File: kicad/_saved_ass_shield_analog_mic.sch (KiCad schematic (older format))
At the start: 151 parts, among them J1 6-40V, J2 DEBUG, J3 5V, J4 UART2, J5 U.FL, J6 i2s, J7 SP, J8 U.FL, M1 CR1220SMD, Q1 BC817, U1 OPiZero, U2 DS3231M, U3 24LC256, U4 nRF24L01P, U5 PCF8574, U6 CC2530F, X1 USB_F1, X2 USB_F1, Y1 9,84375 MHz, Y2 13,5600 MHz, Y3 4,8970 MHz, Y4 6,7458 MHz, Y5 32 MHz, Y6 16 MHz, Y7 32 MHz

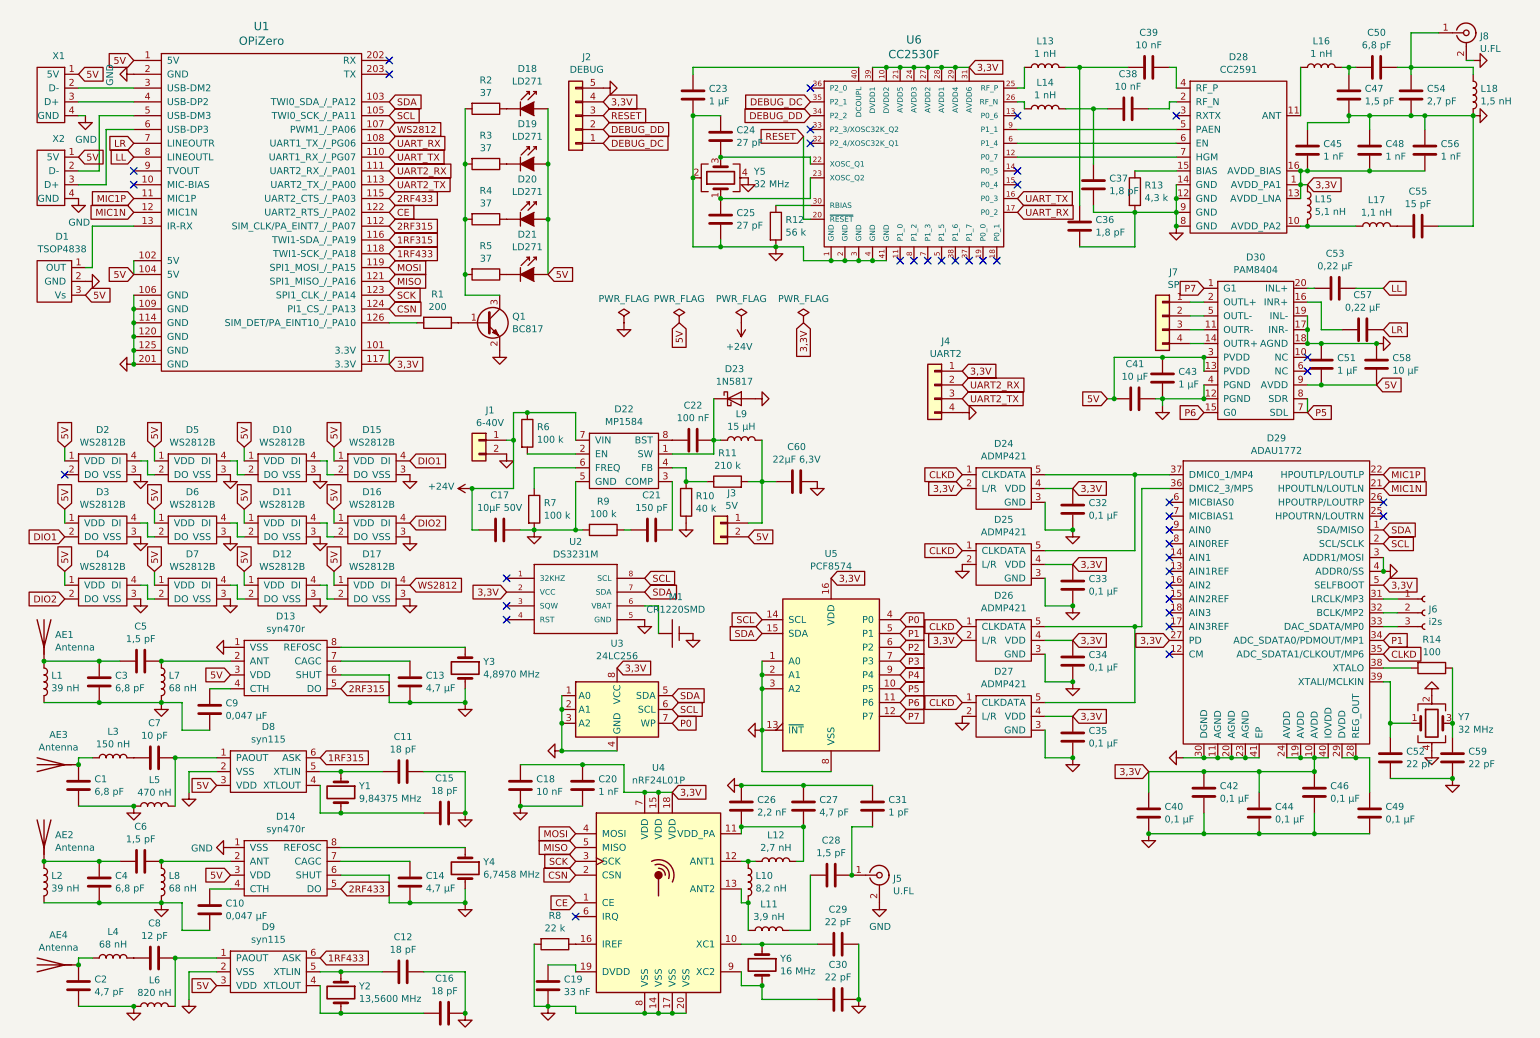
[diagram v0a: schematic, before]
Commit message: Add files via upload
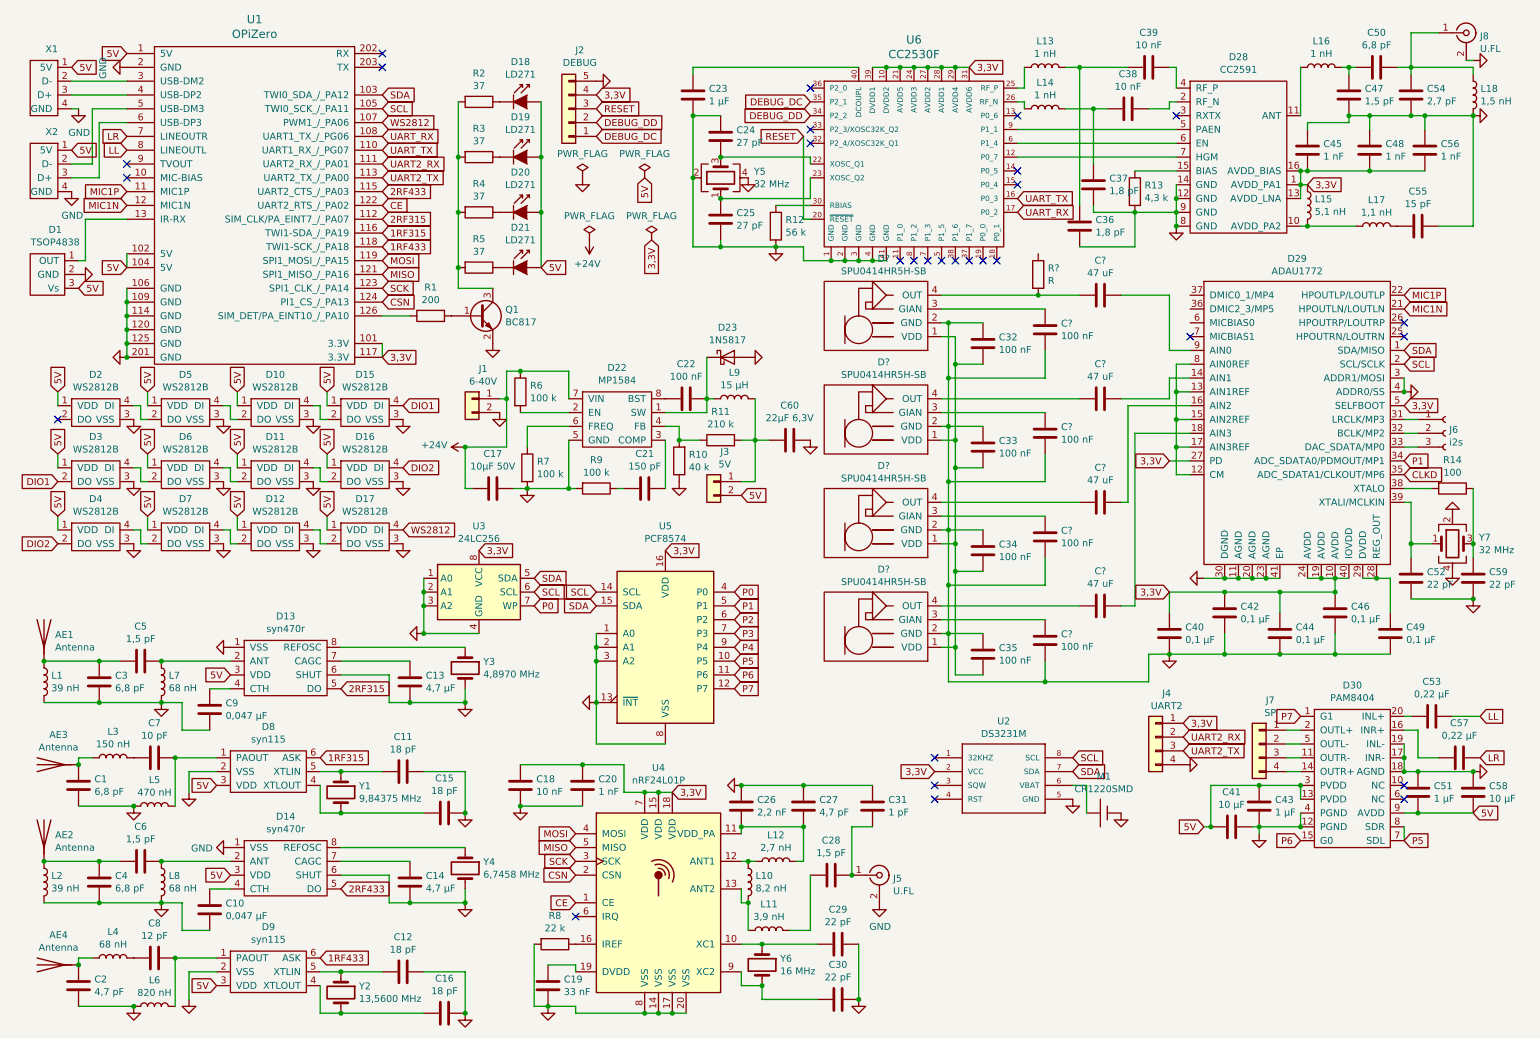
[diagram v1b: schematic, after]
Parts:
- removed D24, D25, D26, D27: ADMP421, imm:ADMP421, symbol ass_shield-rescue:ADMP421-imm_lib
- added C? (x4): 100 nF, Capacitor_SMD:C_0402_1005Metric, symbol ass_shield-rescue:C-imm_lib
- added C? (x4): 47 uF, Capacitor_SMD:C_0402_1005Metric, symbol ass_shield-rescue:C-imm_lib
- added D? (x4): SPU0414HR5H-SB, symbol imm_lib:SPU0414HR5H-SB
- added R?: R, Resistor_SMD:R_0402_1005Metric, symbol imm_lib:R
- C32, C33, C34, C35: value 0,1 µF -> 100 nF
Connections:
- net 3,3V: no longer C32.1, C33.1, C34.1, C35.1
- net GND: now also C32.1, C33.1, C34.1, C35.1, C?.2, C?.2, C?.2, C?.2, D?.2 (GND), D?.2 (GND), D?.2 (GND), D?.2 (GND); no longer C32.2, C33.2, C34.2, C35.2
- net at D29.12 (CM): now also D29.13 (AIN1REF), D29.15 (AIN2REF), D29.17 (AIN3REF), D29.8 (AIN0REF)
- net at D29.14 (AIN1): now also C?.1
- net at D29.16 (AIN2): now also C?.1
- net at D29.18 (AIN3): now also C?.1
- net at D29.9 (AIN0): now also C?.1
- new net: C32.2, C33.2, C34.2, C35.2, D?.1 (VDD), D?.1 (VDD), D?.1 (VDD), D?.1 (VDD)
- new net: C?.1, D?.3 (GIAN) (x4)
- new net: C?.2, D?.4 (OUT), R?.2
- new net: C?.2, D?.4 (OUT) (x3)
- no-connect marks 39 -> 29
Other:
- moved on the sheet: C17, C21, C22, C32, C33, C34, C35, C40, C41, C42, C43, C44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
